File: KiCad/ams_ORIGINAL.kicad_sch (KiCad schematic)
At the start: 4 parts

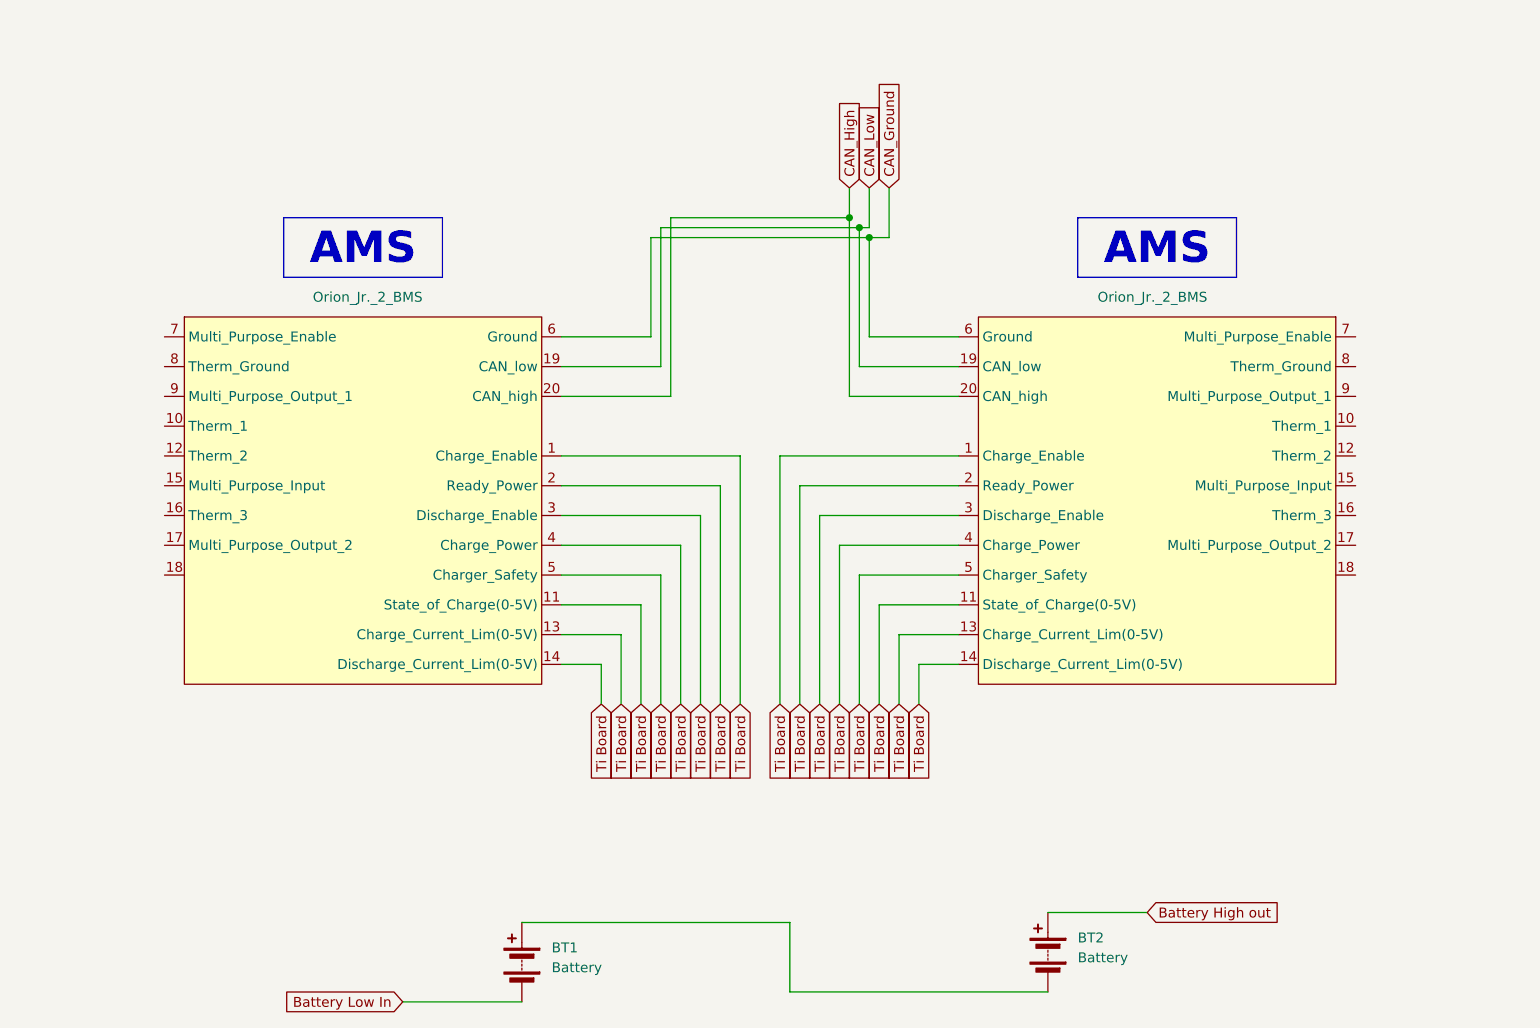
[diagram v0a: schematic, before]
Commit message: 24OCT23
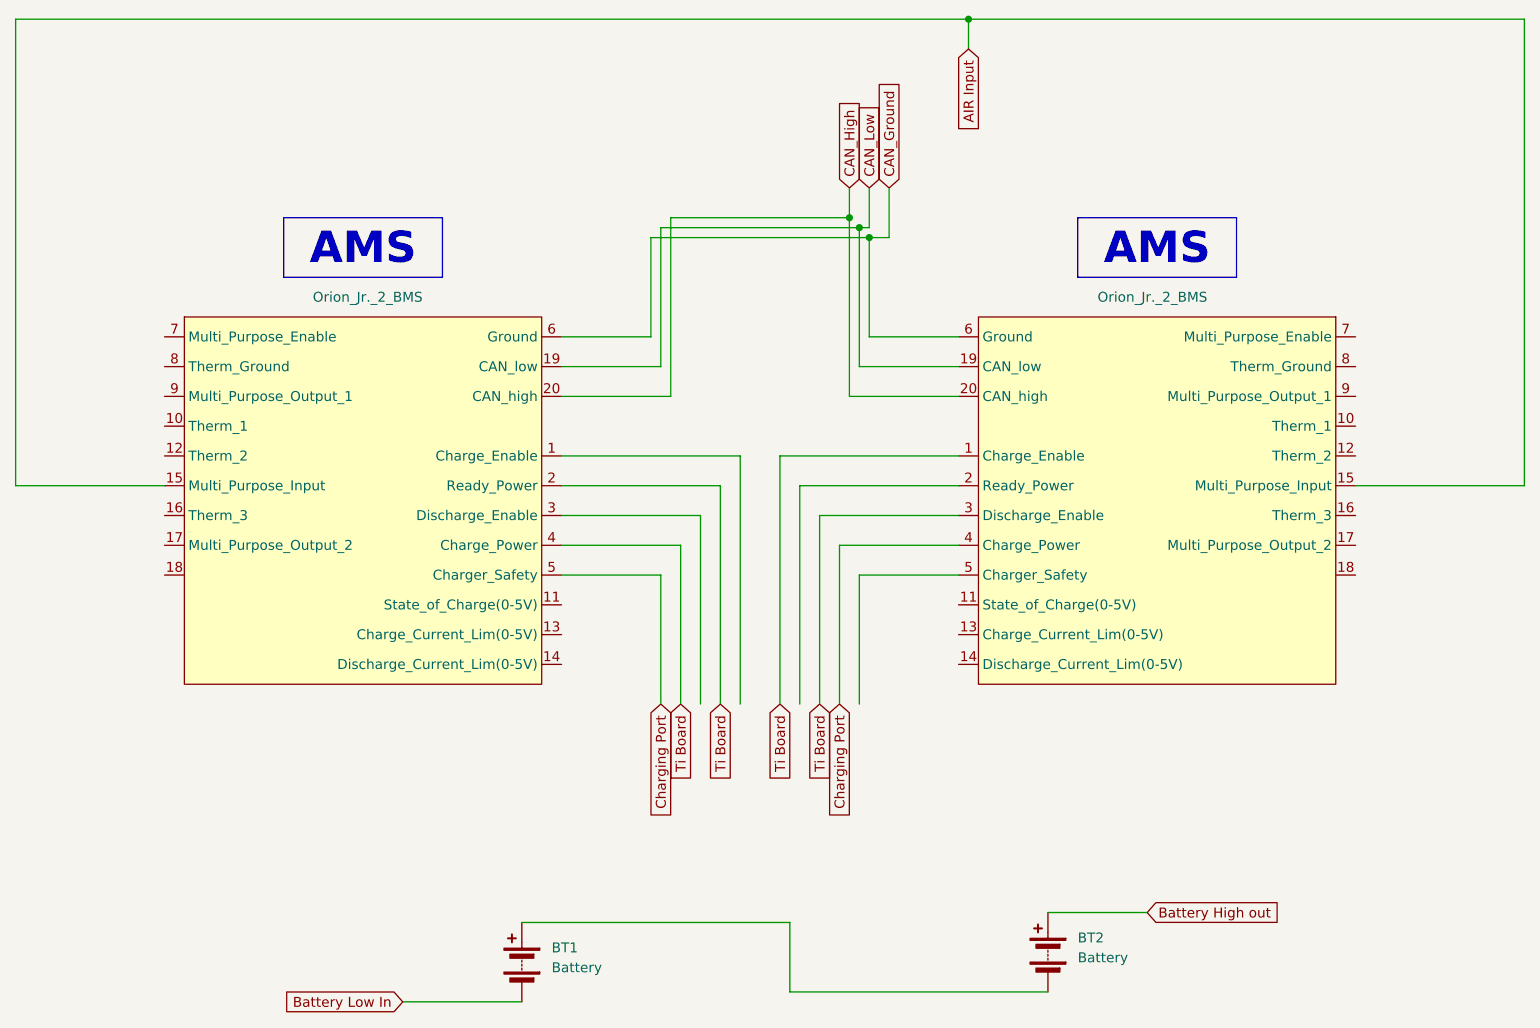
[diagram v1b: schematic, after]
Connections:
- net Ti Board: no longer U?.1 (Charge_Enable), U?.11 (State_of_Charge(0-5V)), U?.11 (State_of_Charge(0-5V)), U?.13 (Charge_Current_Lim(0-5V)), U?.13 (Charge_Current_Lim(0-5V)), U?.14 (Discharge_Current_Lim(0-5V)), U?.14 (Discharge_Current_Lim(0-5V)), U?.2 (Ready_Power), U?.3 (Discharge_Enable), U?.4 (Charge_Power), U?.5 (Charger_Safety), U?.5 (Charger_Safety)
- net AIR Input: now reaches U?.15 (Multi_Purpose_Input)
- net AIR Input: now also U?.15 (Multi_Purpose_Input)
- new net Charging Port: U?.4 (Charge_Power), U?.5 (Charger_Safety)
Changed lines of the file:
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@@
 (kicad_sch (version 20230121) (generator eeschema)
   (paper "A4")
+  (junction (at 182.88 25.4) (diameter 0) (color 0 0 0 0)
+  )
   (junction (at 168.91 52.07) (diameter 0) (color 0 0 0 0)
   )
@@
     (stroke (width 0) (type default))
   )
-  (wire (pts (xy 140.97 100.33) (xy 140.97 113.03))
-    (stroke (width 0) (type default))
-  )
   (wire (pts (xy 181.61 88.9) (xy 163.83 88.9))
     (stroke (width 0) (type default))
@@
     (stroke (width 0) (type default))
   )
-  (wire (pts (xy 171.45 100.33) (xy 171.45 113.03))
+  (wire (pts (xy 80.01 85.09) (xy 60.96 85.09))
     (stroke (width 0) (type default))
   )
@@
     (stroke (width 0) (type default))
   )
+  (wire (pts (xy 254 25.4) (xy 254 85.09))
+    (stroke (width 0) (type default))
+  )
   (wire (pts (xy 181.61 92.71) (xy 166.37 92.71))
     (stroke (width 0) (type default))
@@
     (stroke (width 0) (type default))
   )
-  (wire (pts (xy 130.81 107.95) (xy 135.89 107.95))
-    (stroke (width 0) (type default))
-  )
-  (wire (pts (xy 173.99 104.14) (xy 173.99 113.03))
-    (stroke (width 0) (type default))
-  )
-  (wire (pts (xy 176.53 107.95) (xy 176.53 113.03))
-    (stroke (width 0) (type default))
-  )
   (wire (pts (xy 130.81 88.9) (xy 148.59 88.9))
     (stroke (width 0) (type default))
@@
     (stroke (width 0) (type default))
   )
-  (wire (pts (xy 181.61 100.33) (xy 171.45 100.33))
-    (stroke (width 0) (type default))
-  )
   (wire (pts (xy 130.81 81.28) (xy 153.67 81.28))
     (stroke (width 0) (type default))
   )
-  (wire (pts (xy 181.61 104.14) (xy 173.99 104.14))
+  (wire (pts (xy 254 85.09) (xy 232.41 85.09))
+    (stroke (width 0) (type default))
+  )
+  (wire (pts (xy 60.96 25.4) (xy 182.88 25.4))
     (stroke (width 0) (type default))
   )
@@
     (stroke (width 0) (type default))
   )
-  (wire (pts (xy 130.81 100.33) (xy 140.97 100.33))
-    (stroke (width 0) (type default))
-  )
   (wire (pts (xy 181.61 73.66) (xy 167.64 73.66))
     (stroke (width 0) (type default))
@@
     (stroke (width 1) (type default))
   )
+  (wire (pts (xy 182.88 25.4) (xy 254 25.4))
+    (stroke (width 0) (type default))
+  )
   (wire (pts (xy 170.18 46.99) (xy 170.18 52.07))
     (stroke (width 0) (type default))
@@
     (stroke (width 0) (type default))
   )
+  (wire (pts (xy 182.88 25.4) (xy 182.88 29.21))
+    (stroke (width 0) (type default))
+  )
   (wire (pts (xy 161.29 85.09) (xy 161.29 113.03))
     (stroke (width 0) (type default))
@@
     (stroke (width 0) (type default))
   )
+  (wire (pts (xy 60.96 85.09) (xy 60.96 25.4))
+    (stroke (width 0) (type default))
+  )
   (wire (pts (xy 130.81 69.85) (xy 143.51 69.85))
     (stroke (width 0) (type default))
@@
     (stroke (width 1) (type default))
   )
-  (wire (pts (xy 138.43 104.14) (xy 138.43 113.03))
-    (stroke (width 0) (type default))
-  )
   (wire (pts (xy 144.78 50.8) (xy 167.64 50.8))
     (stroke (width 0) (type default))
@@
     (stroke (width 0) (type default))
   )
-  (wire (pts (xy 135.89 107.95) (xy 135.89 113.03))
-    (stroke (width 0) (type default))
-  )
   (wire (pts (xy 143.51 96.52) (xy 143.51 113.03))
-    (stroke (width 0) (type default))
-  )
-  (wire (pts (xy 130.81 104.14) (xy 138.43 104.14))
-    (stroke (width 0) (type default))
-  )
-  (wire (pts (xy 181.61 107.95) (xy 176.53 107.95))
     (stroke (width 0) (type default))
   )
@@
     (effects (font (size 4 4) (thickness 0.8) bold (color 0 0 0 1)))
   )
-  (global_label "Ti Board" (shape input) (at 143.51 113.03 270) (fields_autoplaced)
-    (effects (font (size 1.27 1.27)) (justify right))
-    (property "Intersheetrefs" "${INTERSHEET_REFS}" (at 143.51 124.0584 90)
-      (effects (font (size 1.27 1.27)) (justify right) hide)
-    )
-  )
-  (global_label "Ti Board" (shape input) (at 171.45 113.03 270) (fields_autoplaced)
-    (effects (font (size 1.27 1.27)) (justify right))
-    (property "Intersheetrefs" "${INTERSHEET_REFS}" (at 171.45 124.0584 90)
+  (global_label "Charging Port" (shape input) (at 143.51 113.03 270) (fields_autoplaced)
+    (effects (font (size 1.27 1.27)) (justify right))
+    (property "Intersheetrefs" "${INTERSHEET_REFS}" (at 143.51 129.3197 90)
       (effects (font (size 1.27 1.27)) (justify right) hide)
     )
@@
     )
   )
-  (global_label "Ti Board" (shape input) (at 161.29 113.03 270) (fields_autoplaced)
-    (effects (font (size 1.27 1.27)) (justify right))
-    (property "Intersheetrefs" "${INTERSHEET_REFS}" (at 161.29 124.0584 90)
-      (effects (font (size 1.27 1.27)) (justify right) hide)
-    )
-  )
-  (global_label "Ti Board" (shape input) (at 135.89 113.03 270) (fields_autoplaced)
-    (effects (font (size 1.27 1.27)) (justify right))
-    (property "Intersheetrefs" "${INTERSHEET_REFS}" (at 135.89 124.0584 90)
-      (effects (font (size 1.27 1.27)) (justify right) hide)
-    )
-  )
-  (global_label "Ti Board" (shape input) (at 173.99 113.03 270) (fields_autoplaced)
-    (effects (font (size 1.27 1.27)) (justify right))
-    (property "Intersheetrefs" "${INTERSHEET_REFS}" (at 173.99 124.0584 90)
-      (effects (font (size 1.27 1.27)) (justify right) hide)
-    )
-  )
-  (global_label "Ti Board" (shape input) (at 138.43 113.03 270) (fields_autoplaced)
-    (effects (font (size 1.27 1.27)) (justify right))
-    (property "Intersheetrefs" "${INTERSHEET_REFS}" (at 138.43 124.0584 90)
-      (effects (font (size 1.27 1.27)) (justify right) hide)
-    )
-  )
-  (global_label "Ti Board" (shape input) (at 140.97 113.03 270) (fields_autoplaced)
-    (effects (font (size 1.27 1.27)) (justify right))
-    (property "Intersheetrefs" "${INTERSHEET_REFS}" (at 140.97 124.0584 90)
-      (effects (font (size 1.27 1.27)) (justify right) hide)
-    )
-  )
   (global_label "Ti Board" (shape input) (at 146.05 113.03 270) (fields_autoplaced)
     (effects (font (size 1.27 1.27)) (justify right))
@@
     )
   )
-  (global_label "Ti Board" (shape input) (at 166.37 113.03 270) (fields_autoplaced)
-    (effects (font (size 1.27 1.27)) (justify right))
-    (property "Intersheetrefs" "${INTERSHEET_REFS}" (at 166.37 124.0584 90)
-      (effects (font (size 1.27 1.27)) (justify right) hide)
-    )
-  )
-  (global_label "Ti Board" (shape input) (at 176.53 113.03 270) (fields_autoplaced)
-    (effects (font (size 1.27 1.27)) (justify right))
-    (property "Intersheetrefs" "${INTERSHEET_REFS}" (at 176.53 124.0584 90)
-      (effects (font (size 1.27 1.27)) (justify right) hide)
+  (global_label "Charging Port" (shape input) (at 166.37 113.03 270) (fields_autoplaced)
+    (effects (font (size 1.27 1.27)) (justify right))
+    (property "Intersheetrefs" "${INTERSHEET_REFS}" (at 166.37 129.3197 90)
+      (effects (font (size 1.27 1.27)) (justify left) hide)
+    )
+  )
+  (global_label "Ti Board" (shape input) (at 163.83 113.03 270) (fields_autoplaced)
+    (effects (font (size 1.27 1.27)) (justify right))
+    (property "Intersheetrefs" "${INTERSHEET_REFS}" (at 163.83 124.0584 90)
+      (effects (font (size 1.27 1.27)) (justify left) hide)
+    )
+  )
+  (global_label "CAN_Low" (shape input) (at 170.18 46.99 90) (fields_autoplaced)
+    (effects (font (size 1.27 1.27)) (justify left))
+    (property "Intersheetrefs" "${INTERSHEET_REFS}" (at 170.18 35.8405 90)
+      (effects (font (size 1.27 1.27)) (justify left) hide)
+    )
+  )
+  (global_label "AIR Input" (shape input) (at 182.88 29.21 270) (fields_autoplaced)
+    (effects (font (size 1.27 1.27)) (justify right))
+    (property "Intersheetrefs" "${INTERSHEET_REFS}" (at 182.88 40.9037 90)
+      (effects (font (size 1.27 1.27)) (justify right) hide)
+    )
+  )
+  (global_label "Battery High out" (shape input) (at 205.74 139.7 0) (fields_autoplaced)
+    (effects (font (size 1.27 1.27)) (justify left))
+    (property "Intersheetrefs" "${INTERSHEET_REFS}" (at 224.6302 139.7 0)
+      (effects (font (size 1.27 1.27)) (justify left) hide)
     )
   )
@@
     (effects (font (size 1.27 1.27)) (justify right))
     (property "Intersheetrefs" "${INTERSHEET_REFS}" (at 158.75 124.0584 90)
-      (effects (font (size 1.27 1.27)) (justify right) hide)
-    )
-  )
-  (global_label "Ti Board" (shape input) (at 168.91 113.03 270) (fields_autoplaced)
-    (effects (font (size 1.27 1.27)) (justify right))
-    (property "Intersheetrefs" "${INTERSHEET_REFS}" (at 168.91 124.0584 90)
-      (effects (font (size 1.27 1.27)) (justify right) hide)
-    )
-  )
-  (global_label "CAN_Low" (shape input) (at 170.18 46.99 90) (fields_autoplaced)
-    (effects (font (size 1.27 1.27)) (justify left))
-    (property "Intersheetrefs" "${INTERSHEET_REFS}" (at 170.18 35.8405 90)
-      (effects (font (size 1.27 1.27)) (justify left) hide)
-    )
-  )
-  (global_label "Ti Board" (shape input) (at 163.83 113.03 270) (fields_autoplaced)
-    (effects (font (size 1.27 1.27)) (justify right))
-    (property "Intersheetrefs" "${INTERSHEET_REFS}" (at 163.83 124.0584 90)
-      (effects (font (size 1.27 1.27)) (justify right) hide)
-    )
-  )
-  (global_label "Battery High out" (shape input) (at 205.74 139.7 0) (fields_autoplaced)
-    (effects (font (size 1.27 1.27)) (justify left))
-    (property "Intersheetrefs" "${INTERSHEET_REFS}" (at 224.6302 139.7 0)
-      (effects (font (size 1.27 1.27)) (justify left) hide)
-    )
-  )
-  (global_label "Ti Board" (shape input) (at 153.67 113.03 270) (fields_autoplaced)
-    (effects (font (size 1.27 1.27)) (justify right))
-    (property "Intersheetrefs" "${INTERSHEET_REFS}" (at 153.67 124.0584 90)
-      (effects (font (size 1.27 1.27)) (justify right) hide)
-    )
-  )
-  (global_label "Ti Board" (shape input) (at 148.59 113.03 270) (fields_autoplaced)
-    (effects (font (size 1.27 1.27)) (justify right))
-    (property "Intersheetrefs" "${INTERSHEET_REFS}" (at 148.59 124.0584 90)
-      (effects (font (size 1.27 1.27)) (justify right) hide)
-    )
-  )
+      (effects (font (size 1.27 1.27)) (justify left) hide)
+    )
+  )
